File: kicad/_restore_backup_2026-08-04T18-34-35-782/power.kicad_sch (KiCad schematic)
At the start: 19 parts, among them J4 2.1mm ID 5.5mm OD PJ-102AH, Q1 DMP3013SFV, U10 TLV75733PDBV, U11 TLV75733PDBV, U9 TPS62163DSG

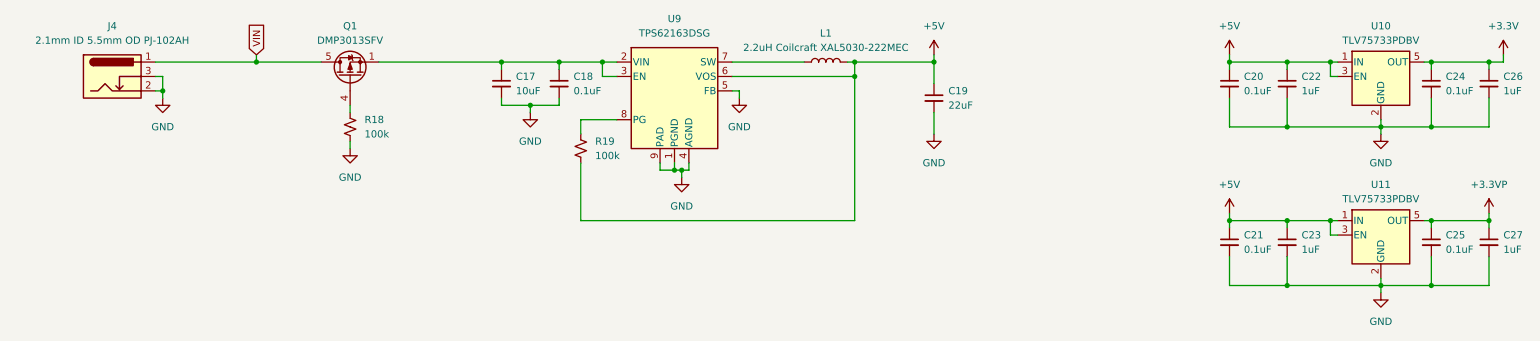
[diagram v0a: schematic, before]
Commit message: finish pcb
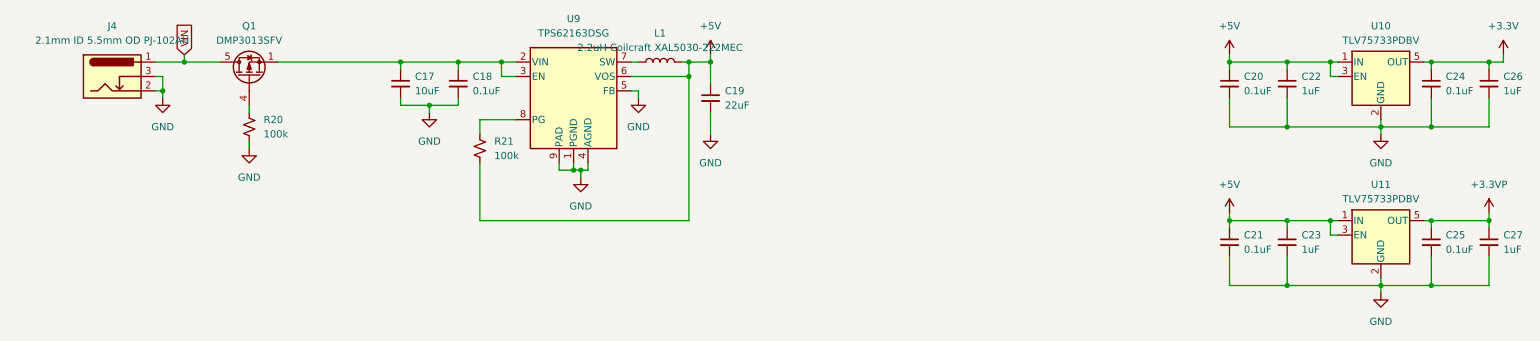
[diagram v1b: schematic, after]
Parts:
- R20: renamed from R18; footprint Resistor_SMD:R_0402_1005Metric -> Resistor_SMD:R_0603_1608Metric
- renumbered R19 to R21
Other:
- moved on the sheet: C17, C18, C19, L1, Q1, R20, R21, U9
